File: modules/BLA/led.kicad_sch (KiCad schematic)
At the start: 3 parts

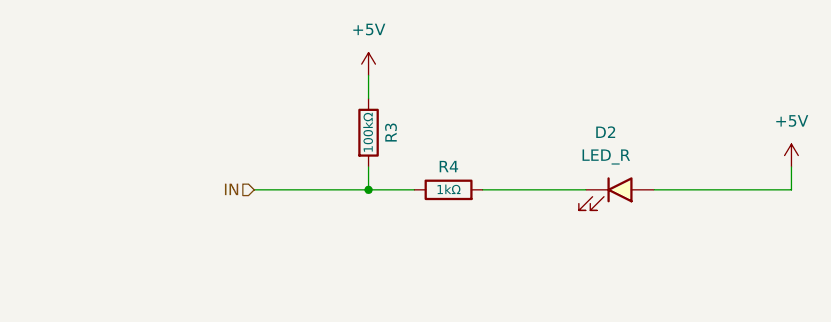
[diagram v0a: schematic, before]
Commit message: minor PW PCB tweaks
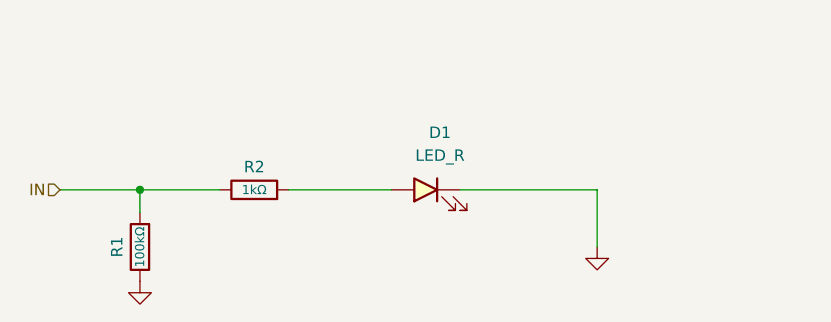
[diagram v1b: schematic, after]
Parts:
- removed D2: LED_R, LED_THT:LED_D3.0mm_Horizontal_O1.27mm_Z2.0mm, symbol IMNOTWOPR:LED_R
- removed R3: 100kΩ, IMNOTWOPR:R_Axial_DIN0207_P400mil, symbol IMNOTWOPR:R
- removed R4: 1kΩ, IMNOTWOPR:R_Axial_DIN0207_P400mil, symbol IMNOTWOPR:R
- added D1: LED_R, LED_THT:LED_D3.0mm_Horizontal_O1.27mm_Z2.0mm, symbol IMNOTWOPR:LED_R
- added R1: 100kΩ, IMNOTWOPR:R_Axial_DIN0207_P400mil, symbol IMNOTWOPR:R
- added R2: 1kΩ, IMNOTWOPR:R_Axial_DIN0207_P400mil, symbol IMNOTWOPR:R
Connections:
- net IN: now also R1.2, R2.1
- new net: D1.2 (A), R2.2
- new net GND: D1.1 (K), R1.1
